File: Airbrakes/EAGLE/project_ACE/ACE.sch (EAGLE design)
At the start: 7 parts, among them J2 SMD, J3 PTH, J4 SMD

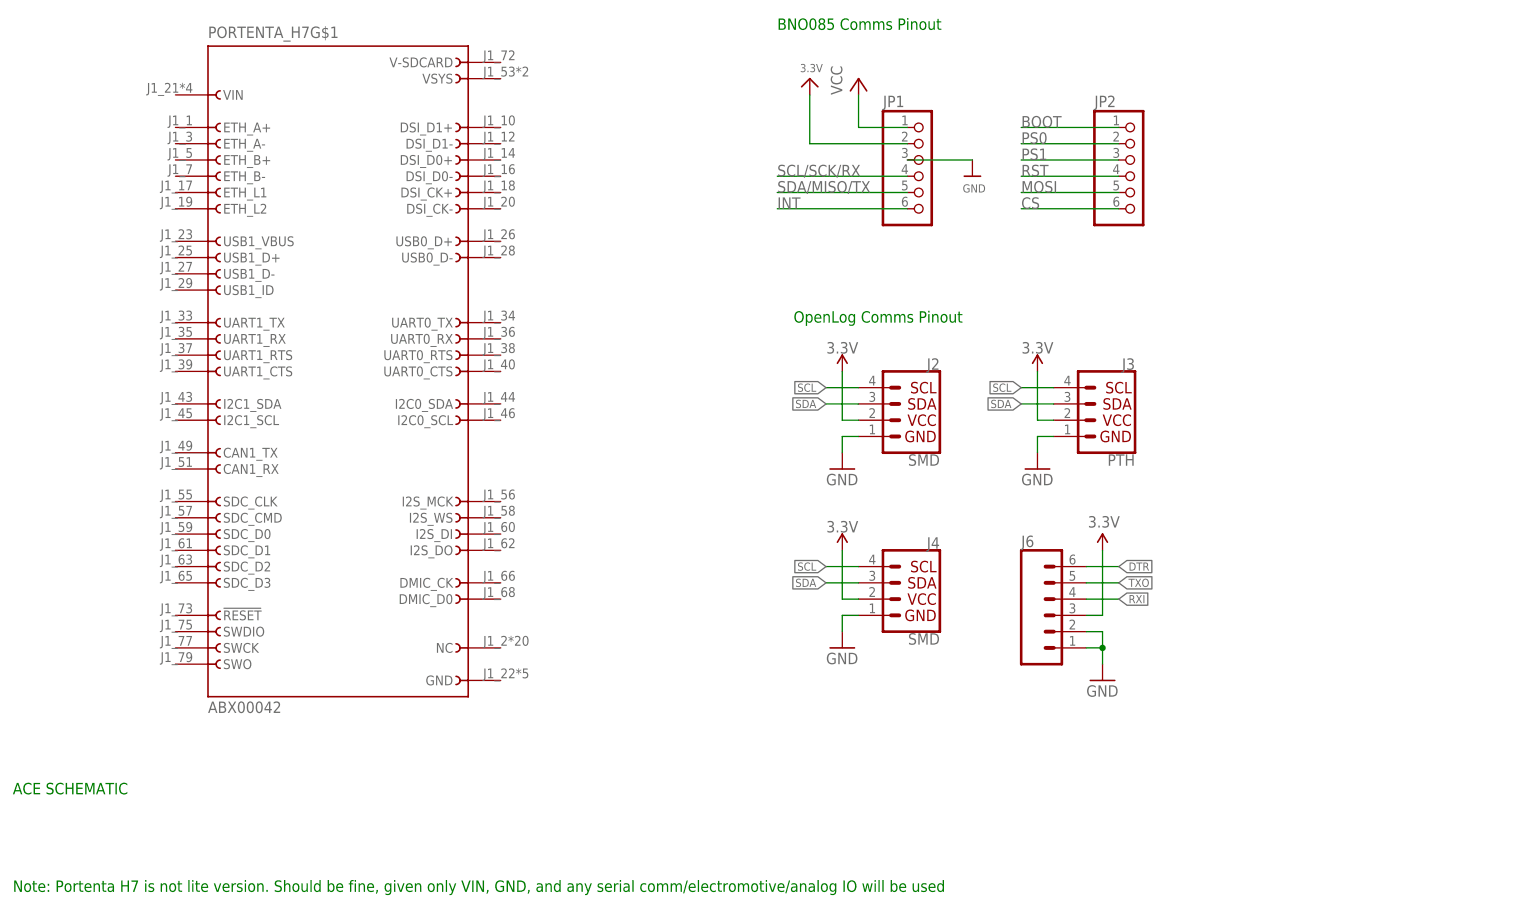
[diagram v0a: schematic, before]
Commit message: Fix version
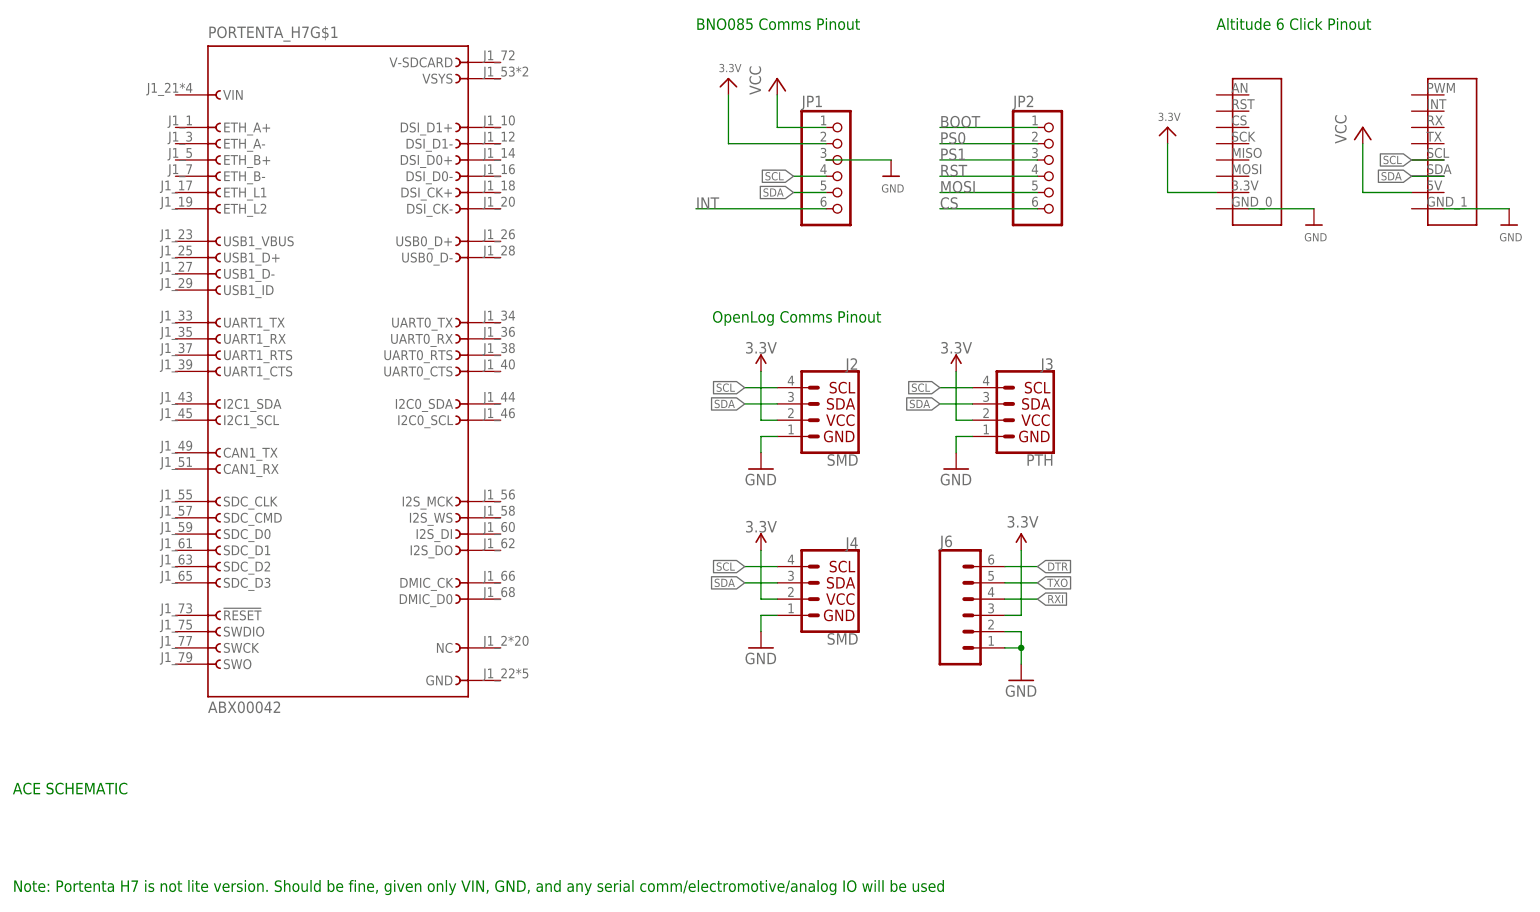
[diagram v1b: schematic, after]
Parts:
- added U$1: MIKROE-ALTITUDE-6-CLICK-DVC, MIKROE-4903:MIKROE-ALTITUDE-6-CLICK-DVC
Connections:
- removed net SCL/SCK/RX: JP1.4
- removed net SDA/MISO/TX: JP1.5
- net GND: now also U$1.GND_0, U$1.GND_1
- net SCL: now also JP1.4, U$1.SCL
- net SDA: now also JP1.5, U$1.SDA
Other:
- note added: "Altitude 6 Click Pinout"
- moved on the sheet: J2, J3, J4, J6, JP1, JP2
